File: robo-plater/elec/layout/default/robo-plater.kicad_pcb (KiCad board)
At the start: 2 copper layers, 238 parts, among them J1 ?, J2 ?, J3 ?, J4 ?, J5 ?, J6 ?, J7 ?, J8 ?, U1 ?, U10 ?, U11 ?, U12 ?, U13 ?, U14 ?, U15 ?, U16 ?, U17 ?, U18 ?, U19 ?, U2 ?, U20 ?, U21 ?, U22 ?, U23 ?, U24 ?, U25 ?, U26 ?, U27 ?, U28 ?, U29 ?, U3 ?, U30 ?, U31 ?, U32 ?, U33 ?, U34 ?, U35 ?, U36 ?, U37 ?, U38 ?, U39 ?, U4 ?, U40 ?, U41 ?, U42 ?, U43 ?, U44 0.6A, 42V, 1.1MHz Buck Regula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, U45 ?, U46 ?, U47 ?, U48 ?, U49 ?, U5 ?, U50 ?, U51 ?, U6 ?, U7 ?, U8 ?, U9 ?

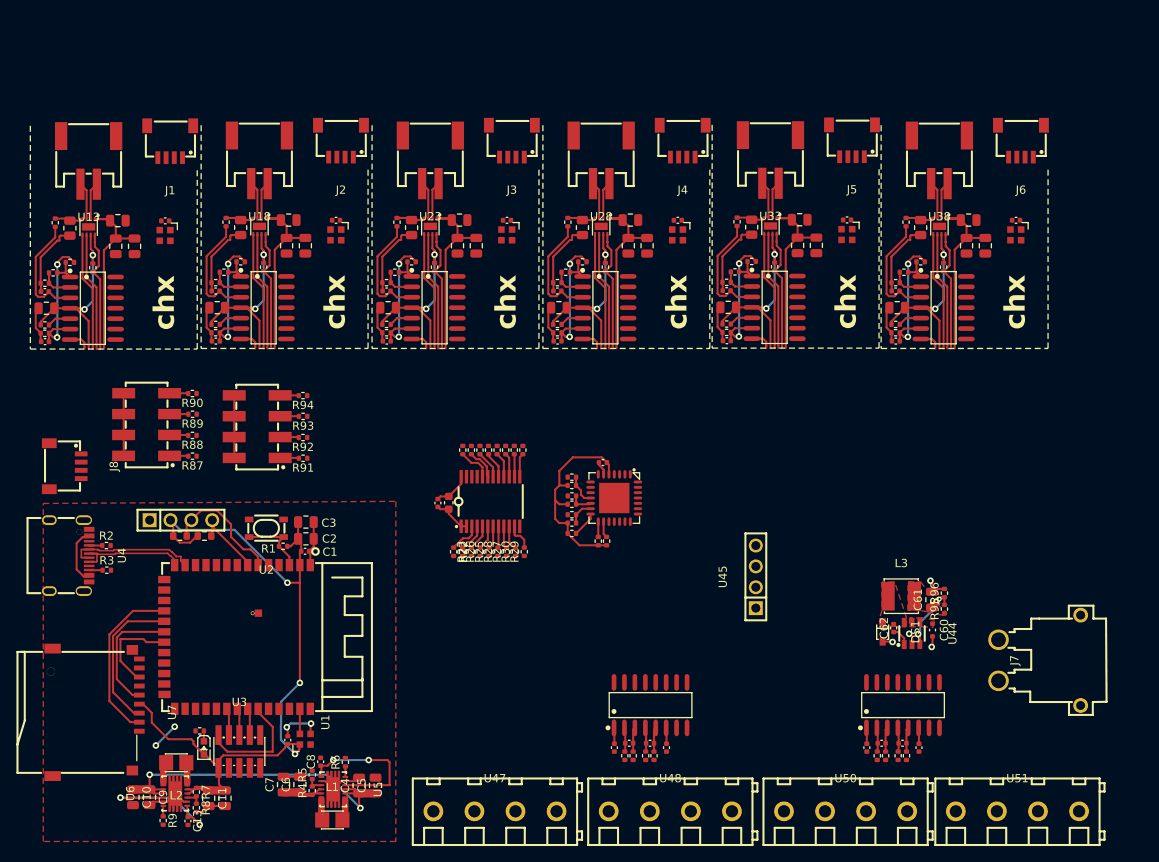
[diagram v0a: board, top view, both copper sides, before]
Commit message: Layout v0.1 done
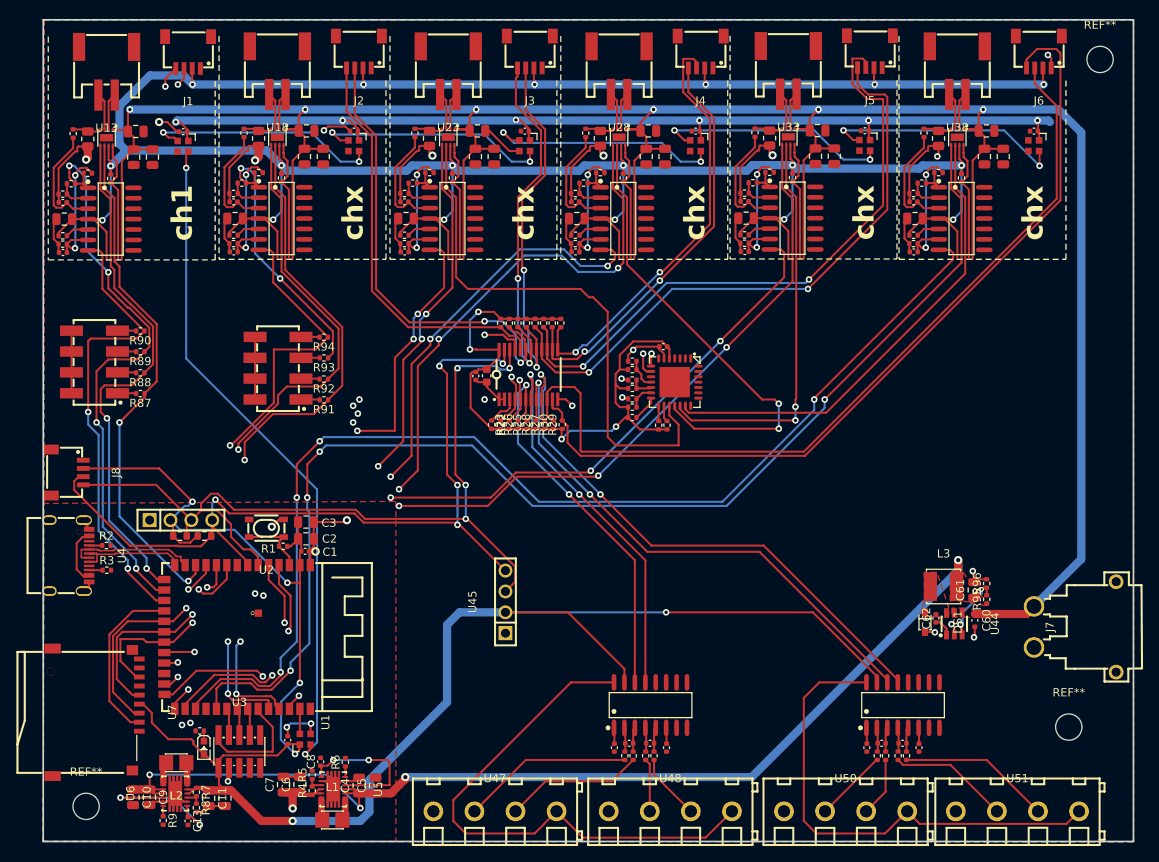
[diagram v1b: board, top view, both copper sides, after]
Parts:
- added REF**: MountingHole_3.2mm_M3, MountingHole:MountingHole_3.2mm_M3, F.Cu at (161.3, 40.1)
- added REF**: MountingHole_3.2mm_M3, MountingHole:MountingHole_3.2mm_M3, F.Cu at (37.8, 131.1)
- added REF**: MountingHole_3.2mm_M3, MountingHole:MountingHole_3.2mm_M3, F.Cu at (157.5, 121.4)
- R5: value 62.5mW Thick Film Resistors 50V ±1% ±200ppm/℃ 2.8kΩ 0402 Chip Resistor - Surface Mount ROHS -> 62.5mW Thick Film Resistors 50V ±100ppm/℃ ±1% 2.8kΩ 0402 Chip Resistor - Surface Mount ROHS
- moved U45 30.6 mm to (88.9, 106.2)
- moved C16 16.1 mm to (85.3, 78.7)
- moved R23 16.1 mm to (89.4, 84.6)
- moved R25 16.1 mm to (91.5, 84.6)
- moved R31 16.1 mm to (94.6, 72.2)
- moved R37 16.1 mm to (88.3, 72.2)
- moved R38 16.1 mm to (89.4, 72.2)
- moved U11 16.1 mm to (91.7, 78.5)
- moved C17 16.1 mm to (86.6, 78.6)
- moved R22 16.1 mm to (87.2, 84.6)
- moved R24 16.1 mm to (88.3, 84.6)
- moved R26 16.1 mm to (90.4, 84.6)
- moved R27 16.1 mm to (93.7, 84.6)
- moved R28 16.1 mm to (92.6, 84.6)
- moved R29 16.1 mm to (95.8, 84.6)
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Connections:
- J2 pad 3: i2c_mux.ic-sda-1 -> i2c_mux.ic-sda-7
- J2 pad 4: i2c_mux.ic-scl-1 -> i2c_mux.ic-scl-7
- J3 pad 3: i2c_mux.ic-sda-2 -> i2c_mux.ic-sda-6
- J3 pad 4: i2c_mux.ic-scl-2 -> i2c_mux.ic-scl-6
- J4 pad 3: i2c_mux.ic-sda-3 -> i2c_mux.ic-sda-4
- J4 pad 4: i2c_mux.ic-scl-3 -> i2c_mux.ic-scl-4
- J5 pad 3: i2c_mux.ic-sda-4 -> i2c_mux.ic-sda-5
- J5 pad 4: i2c_mux.ic-scl-4 -> i2c_mux.ic-scl-5
- J6 pad 3: i2c_mux.ic-sda-5 -> i2c_mux.ic-sda-3
- J6 pad 4: i2c_mux.ic-scl-5 -> i2c_mux.ic-scl-3
- U1 pad 10: ch2.pulses -> ch2.dir
- U1 pad 11: ch2.current -> ch2.pulses
- U1 pad 12: ch2.dir -> ch1.dir
- U1 pad 15: ch2.pwm -> ch1.pwm
- U1 pad 16: ch3.pulses -> ch1.current
- U1 pad 17: io9 -> ch1.pulses
- U1 pad 37: txd0 -> ch3.pulses
- U1 pad 4: ch1.pulses -> io4
- U1 pad 5: ch1.current -> io5
- U1 pad 8: ch1.dir -> io15
- U1 pad 9: ch1.pwm -> ch2.pwm
- U46 pad 13: i2c_mux.ic-scl-6 -> i2c_mux.ic-scl-1
- U46 pad 14: i2c_mux.ic-sda-6 -> i2c_mux.ic-sda-1
- U49 pad 13: i2c_mux.ic-scl-7 -> i2c_mux.ic-scl-2
- U49 pad 14: i2c_mux.ic-sda-7 -> i2c_mux.ic-sda-2
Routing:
- net vcc-2: track 263.2 -> 750.3 mm, vias 15 -> 28
- net vcc-1: track 6.20 -> 231.4 mm, vias 0 -> 7
- net vcc: track 136.2 -> 338.6 mm, vias 0 -> 6
- net ch6.pulses: track 2.68 -> 139.9 mm, vias 0 -> 4
- net ch6.pwm: track 14.4 -> 150.6 mm, vias 0 -> 4
- net uc.uc.ic-sda: track 9.25 -> 126.9 mm, vias 0 -> 6
- net uc.uc.ic-scl: track 15.0 -> 128.3 mm, vias 0 -> 5
- net ch5.pwm: track 14.4 -> 121.9 mm, vias 0 -> 4
- net ch5.pulses: track 2.68 -> 110.2 mm, vias 0 -> 4
- net i2c_mux.ic-scl-3: track 3.42 -> 103.7 mm
- net i2c_mux.ic-sda-3: track 2.94 -> 103.3 mm
- net ch4.pwm: track 14.4 -> 109.5 mm, vias 0 -> 4
- net ch4.pulses: track 2.68 -> 94.6 mm, vias 0 -> 4
- net uc-vcc: track 42.3 -> 129.1 mm, vias 2 -> 4
- net uc._led.ic-led_dout: track 0.00 -> 82.1 mm, vias 0 -> 2
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- added copper zone on B.Cu, net gnd
- added copper zone on In1.Cu, net gnd
- added copper zone on In2.Cu, net gnd
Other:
- board outline added: 132.7 x 100 mm
- copper layers 2 -> 4
- board text added: "ch1"
